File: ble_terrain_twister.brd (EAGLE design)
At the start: 26.8 x 15.5 mm, 14 parts, among them IC1 UA78M33DCY

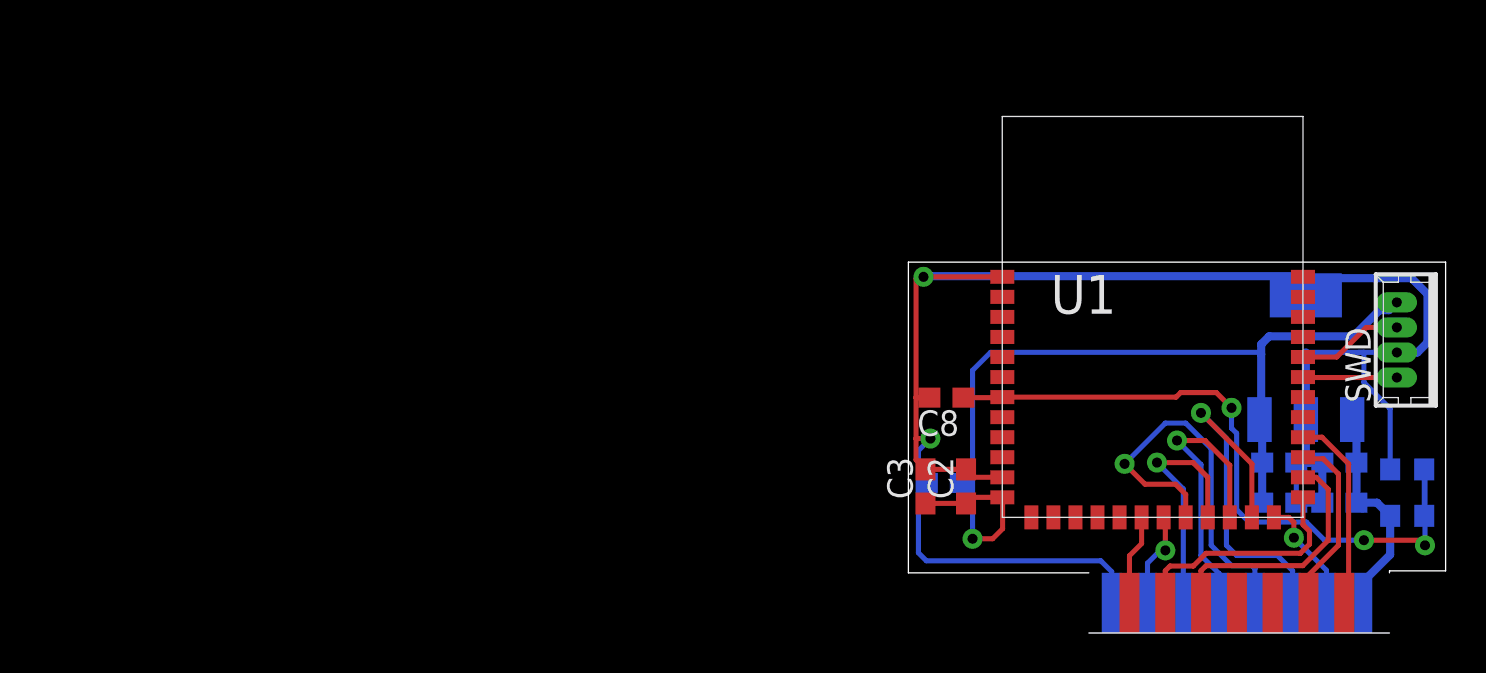
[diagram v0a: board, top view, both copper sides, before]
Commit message: Finished routing. again.
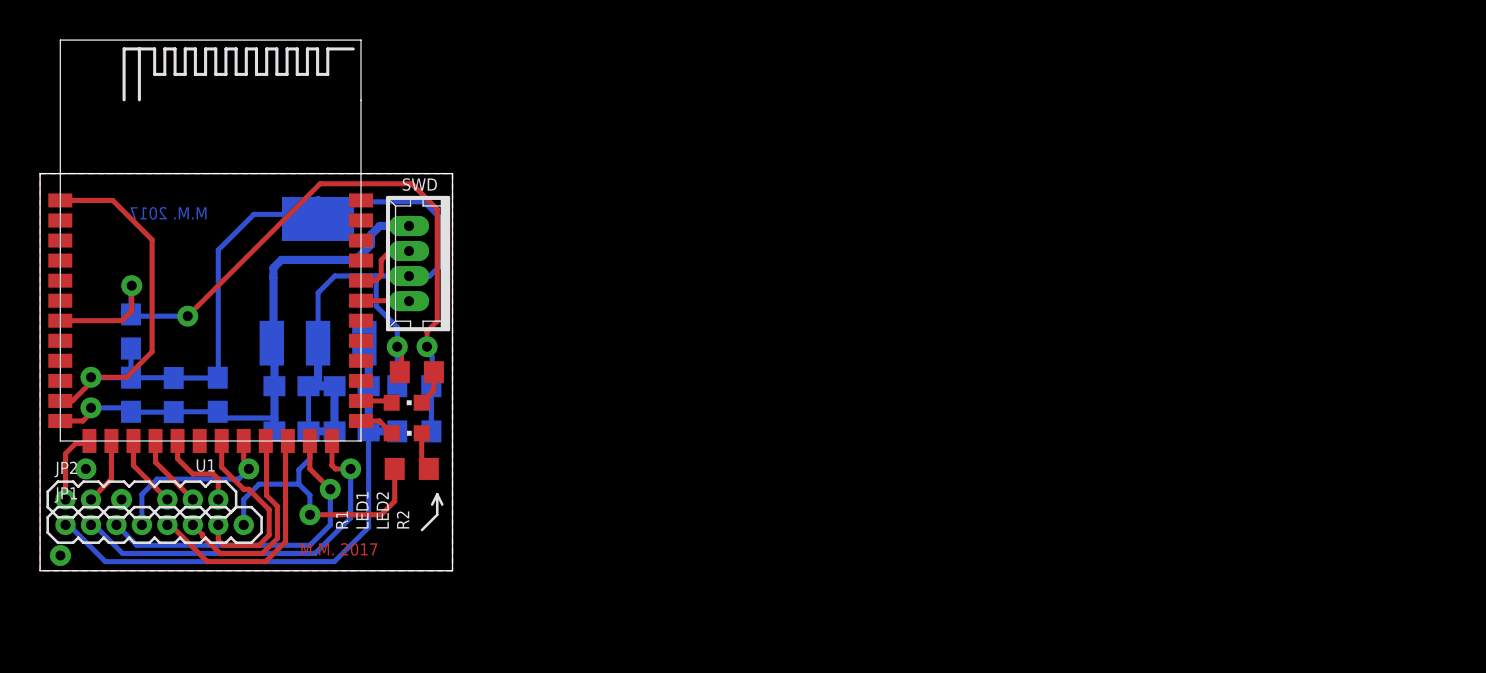
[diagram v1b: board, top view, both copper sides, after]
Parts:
- removed BRD1: TERRAIN_TWISTER_EDGEEDGE, terrain_twister_control_board_edge:TERRAIN_TWISTER_CONTROL_BRD_EDGE
- added JP1: (no value), SparkFun:1X08_1.27MM
- added JP2: LEFT_PH, terrain_twister_control_board_edge:1X08_1.27MM
- added LED1, LED2: LED0603, CEDT:CHIPLED_0603
- added R1, R2: 100, rcl:R0603
- U1: value (none) -> YJ-14015
- moved R6 49.7 mm to (30.4, 13.6)
- moved R7 49.7 mm to (30.4, 15.8)
- moved IC1 49.4 mm to (25.6, 21.1)
- moved SWD 49.4 mm to (30.5, 21.9)
- moved C4 49.4 mm to (24.2, 15.8)
- moved C6 49.4 mm to (27.2, 15.8)
- moved C5 49.4 mm to (24.2, 13.6)
- moved C7 49.4 mm to (27.2, 13.6)
- moved U1 47.1 mm to (20.2, 13.1)
- moved C2 41.9 mm to (16.2, 15.4), flipped to the bottom
- moved C8 40.8 mm to (16.2, 18.5), flipped to the bottom, turned to 270 degrees
- moved C1 38.7 mm to (18.4, 15.4), turned to 90 degrees
- moved C3 35.6 mm to (20.5, 15.4), flipped to the bottom
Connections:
- new net N$1: LED1.C, R1.2
- new net N$2: LED2.C, R2.2
- new net STATUS_LED_A: LED1.A, U1.P.11
- new net STATUS_LED_B: LED2.A, U1.P.12
- net A: now also JP1.4; no longer BRD1.5
- net B: now also JP2.7, U1.P.03; no longer BRD1.15, U1.P.04
- net C: now also JP1.7; no longer BRD1.2
- net GND: now also JP1.8, R1.1, R2.1; no longer BRD1.1
- net M1+: now also JP2.6, U1.P.02; no longer BRD1.14, U1.P.11
- net M1-: now also JP2.5, U1.P.01; no longer BRD1.13, U1.P.12
- net M2+: now also JP1.2; no longer BRD1.7
- net M2-: now also JP1.3; no longer BRD1.6
- net M3+: now also JP1.5; no longer BRD1.4
- net M3-: now also JP1.6; no longer BRD1.3
- net SW2: now also JP2.2, U1.P.00; no longer BRD1.10, U1.P.13
- net SW3: now also JP2.1, U1.P.30; no longer BRD1.9, U1.P.14
- net VBAT: now also JP1.1; no longer BRD1.8
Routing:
- net VCC: track 47.3 -> 28.3 mm
- net VBAT: track 11.8 -> 27.8 mm
- net M2+: track 5.79 -> 18.9 mm
- net A: track 19.7 -> 8.88 mm
- net M1-: track 12.6 -> 3.62 mm
- net M1+: track 11.8 -> 3.69 mm
- net SW3: track 9.86 -> 3.74 mm
- net SW2: track 9.17 -> 3.34 mm
- net C: track 4.82 -> 9.44 mm, vias 1 -> 0
- net M2-: track 18.9 -> 16.1 mm
- net M3+: track 14.7 -> 12.2 mm, vias 1 -> 0
- net SWDIO: track 4.69 -> 2.41 mm
- net M3-: track 12.4 -> 10.3 mm, vias 1 -> 0
- net N$1: track 0.00 -> 1.92 mm
- net SWDCLK: track 5.29 -> 3.45 mm
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- added copper zone on layer 1, net GND
- added copper zone on layer 16, net GND
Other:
- board size 26.8 x 15.5 mm -> 20.6 x 19.8 mm
- board text added: "M.M. 2017"
- board text removed: "Daughterboard key slot"
- board text removed: "Factory PCB top"
